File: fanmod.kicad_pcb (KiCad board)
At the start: 2 copper layers, 15 x 15 mm, 6 parts, among them J1 FAN_IN, J2 FAN_OUT, J4 COMM

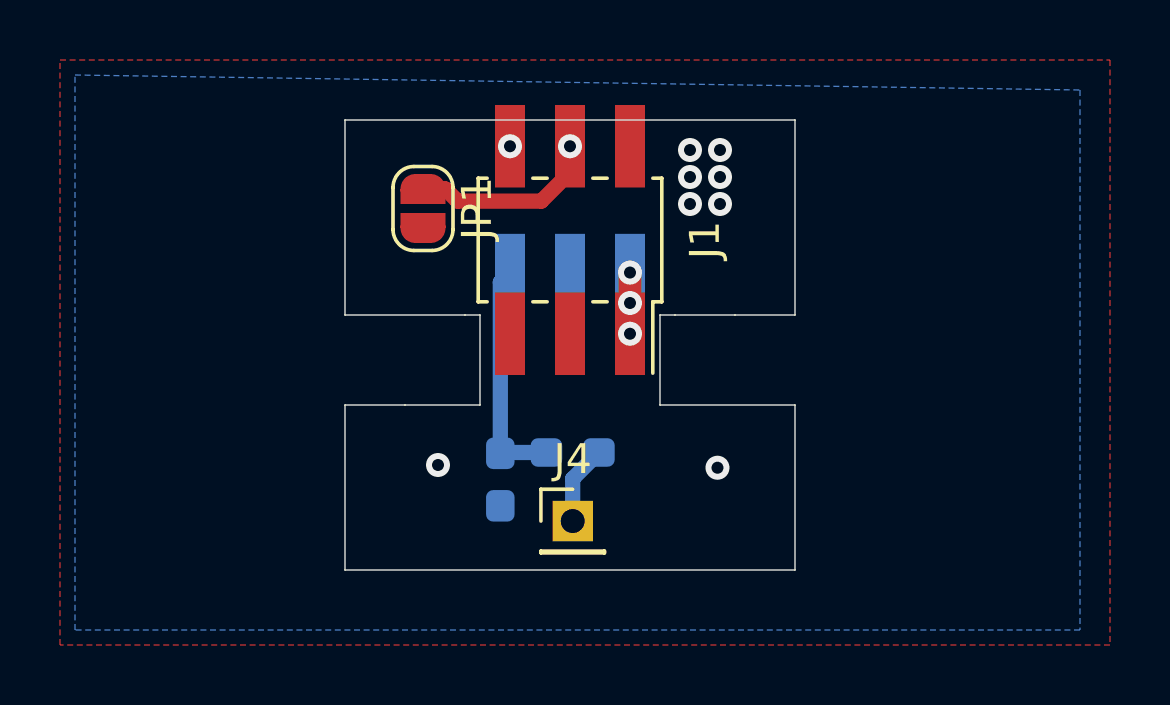
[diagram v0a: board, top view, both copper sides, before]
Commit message: dl380e board 2.0
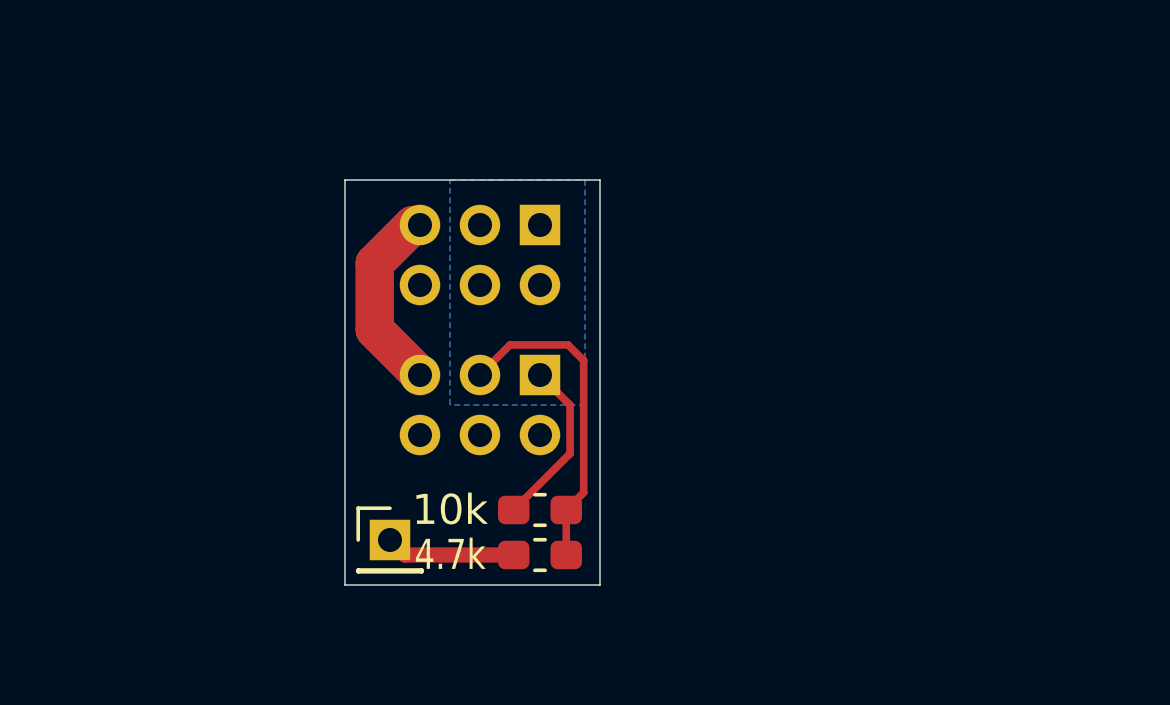
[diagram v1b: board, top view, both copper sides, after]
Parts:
- removed JP1: BYPASS, Jumper:SolderJumper-2_P1.3mm_Open_RoundedPad1.0x1.5mm
- J1: footprint Connector_PinSocket_2.00mm:PinSocket_2x03_P2.00mm_Vertical_SMD -> Connector_PinSocket_2.00mm:PinSocket_2x03_P2.00mm_Vertical; moved to B.Cu
- J2: footprint Connector_PinHeader_2.00mm:PinHeader_2x03_P2.00mm_Vertical_SMD -> Connector_PinSocket_2.00mm:PinSocket_2x03_P2.00mm_Vertical
- R1: value 1k -> 4.7k; moved to F.Cu
- R2: value 2k -> 10k; moved to F.Cu
- moved J4 6.12 mm to (79.0, 32.0)
- moved J2 5.59 mm to (84.0, 26.5)
- moved R1 3.59 mm to (84.0, 32.5), turned to 0 degrees
- moved R2 1.67 mm to (84.0, 31.0), turned to 180 degrees
- moved J1 1.12 mm to (84.0, 21.5), turned to 90 degrees
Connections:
- J1 pad 1: +12V -> GND
- J1 pad 4: GROUND_LOOP -> GND
- J1 pad 5: (no net) -> +12V
- J1 pad 6: ROTATION_DETECT -> (no net)
- J2 pad 1: +12V -> GND
- J2 pad 2: GND -> (no net)
- J2 pad 3: (no net) -> Net-(J2-Pad3)
- J2 pad 4: GROUND_LOOP -> (no net)
- J2 pad 5: Net-(J2-Pad5) -> +12V
- J2 pad 6: ROTATION_DETECT -> (no net)
- R1 pad 2: Net-(J2-Pad5) -> Net-(J2-Pad3)
- R2 pad 1: Net-(J2-Pad5) -> Net-(J2-Pad3)
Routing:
- net Net-(J2-Pad3): track 0.00 -> 10.8 mm
- net +12V: track 4.08 -> 12.8 mm, vias 3 -> 0
- net Net-(J2-Pad5): track 7.71 -> 0.00 mm
- net GROUND_LOOP: track 6.34 -> 0.00 mm, vias 1 -> 0
- net GND: track 0.00 -> 5.69 mm, vias 8 -> 0
- net Net-(J4-Pad1): track 2.65 -> 4.33 mm
- net ROTATION_DETECT: track 0.04 -> 0.00 mm, vias 1 -> 0
- removed copper zone on F.Cu, net GND
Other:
- board size 15 x 15 mm -> 8.5 x 13.5 mm
